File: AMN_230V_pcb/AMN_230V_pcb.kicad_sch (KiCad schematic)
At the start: 37 parts, among them J1 Screw_Terminal_01x03, J2 Screw_Terminal_01x03, J3 Screw_Terminal_01x03, J4 Screw_Terminal_01x04, J5 Conn_02x04_Odd_Even, J6 Screw_Terminal_01x04, K1 Relay_SPST-NO, K2 Relay_SPST-NO, K3 Relay_SPST-NO, Q1 BC817, Q2 BC817, Q3 BC817, T1 TRANSF1, U1 7812

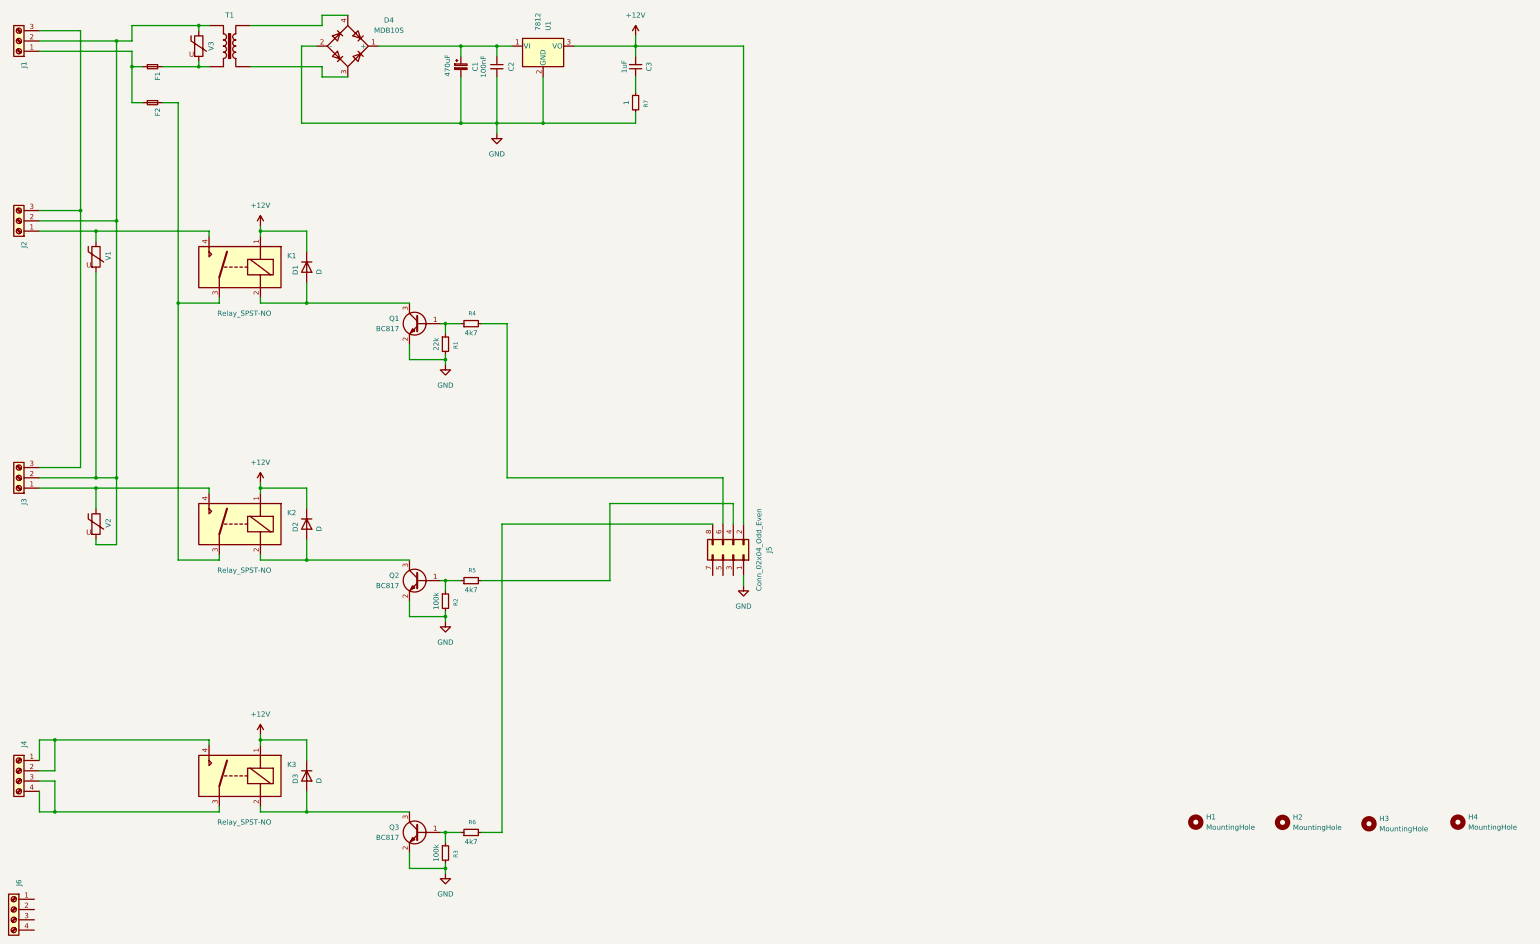
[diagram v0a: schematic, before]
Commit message: 2
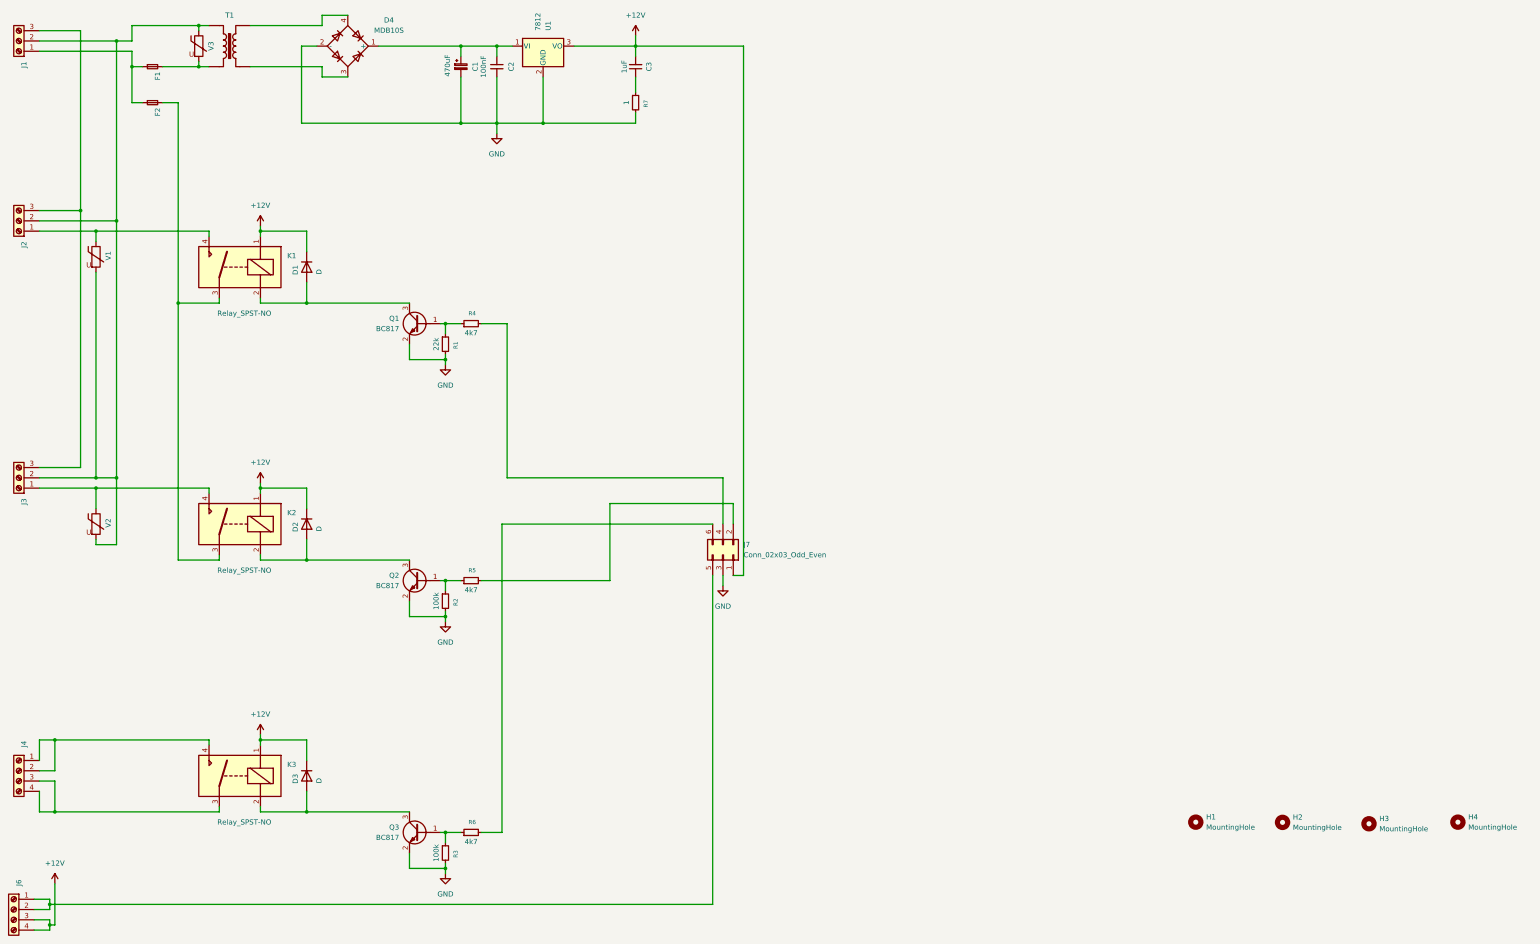
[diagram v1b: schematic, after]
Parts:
- removed J5: Conn_02x04_Odd_Even, Connector_PinSocket_2.54mm:PinSocket_2x04_P2.54mm_Vertical, symbol Connector_Generic:Conn_02x04_Odd_Even
- added J7: Conn_02x03_Odd_Even, Connector_PinSocket_2.54mm:PinSocket_2x03_P2.54mm_Vertical, symbol Connector_Generic:Conn_02x03_Odd_Even
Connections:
- net +12V: now also J6.3 (Pin_3), J6.4 (Pin_4), J7.1 (Pin_1)
- net GND: now also J7.3 (Pin_3)
- net at R4.2: now also J7.4 (Pin_4)
- net at J6.1 (Pin_1): now also J6.2 (Pin_2), J7.5 (Pin_5)
- net at R6.2: now also J7.6 (Pin_6)
- net at R5.2: now also J7.2 (Pin_2)
